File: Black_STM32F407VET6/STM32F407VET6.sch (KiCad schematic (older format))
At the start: 89 parts, among them J1 T0, J10 - HotBed +, J11 Heater0, J12 X-, J13 Y-, J14 Z-, J15 Z+, J16 USB_B, J17 LeftSpi, J18 EXTRAPINS, J19 12Vinput, J2 T1, J20 5VOut, J23 EXP2, J24 LCD2004, J25 Bottom, J26 Right, J28 LIGHTS, J29 Z, J3 TB, J30 Z, J38 X, J39 Y, J4 TC, J41 E0, J43 Heater1, J44 COM, J47 I2C, J48 SPI, J49 SPI, J5 + VIN -, J50 SDIO, J51 Servo, J52 Servo, J53 PowerSelect, J54 Power, J55 PD11, J56 Power, J6 Fan3, J7 Fan2, J8 Fan1, J9 Fan0, Q12 IRLR8726PBF, Q13 IRLR8726PBF, Q14 IRLR8726PBF, Q4 IRLML0030TRPBF, Q6 IRLML0030TRPBF, Q7 IRLML0030TRPBF, Q8 IRLML0030TRPBF, SW1 Boot0, U1 LeftAnalog, U2 Left5V, U3 BuckConvertor, U4 LM2901, U5 AT24CS01-SSHM, U6 LM2901

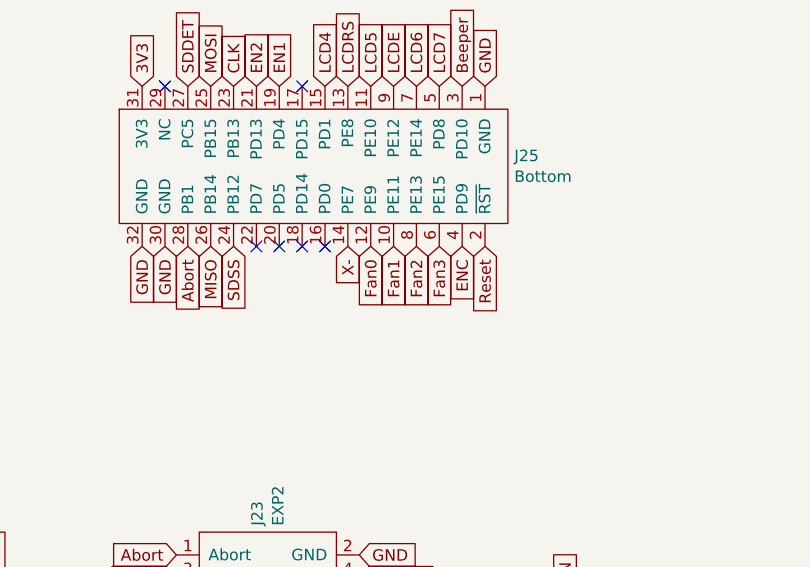
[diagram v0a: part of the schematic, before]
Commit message: Board layout with the opamps
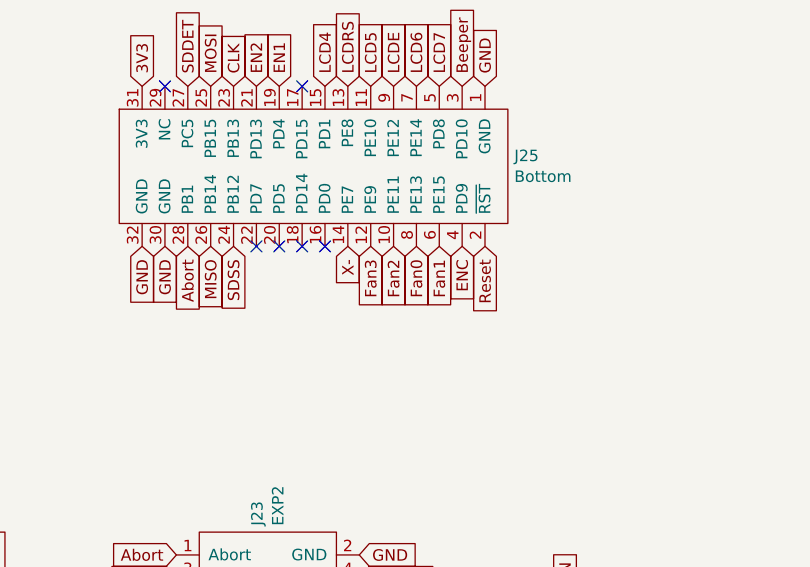
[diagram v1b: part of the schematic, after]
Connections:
- net Fan0: now also J25.8 (PE13); no longer J25.12 (PE9)
- net Fan1: now also J25.6 (PE15); no longer J25.10 (PE11)
- net Fan2: now also J25.10 (PE11); no longer J25.8 (PE13)
- net Fan3: now also J25.12 (PE9); no longer J25.6 (PE15)
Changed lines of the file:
@@
 EESchema Schematic File Version 4
 LIBS:STM32F407VET6-cache
-EELAYER 30 0
+EELAYER 29 0
 EELAYER END
 $Descr A3 16535 11693
@@
 Text GLabel 10700 4900 1    50   Input ~ 0
 3V3
+Text GLabel 11900 5600 3    50   Input ~ 0
+Fan0
+Text GLabel 12000 5600 3    50   Input ~ 0
+Fan1
+Text GLabel 11800 5600 3    50   Input ~ 0
+Fan2
 Text GLabel 11700 5600 3    50   Input ~ 0
-Fan0
-Text GLabel 11800 5600 3    50   Input ~ 0
-Fan1
-Text GLabel 11900 5600 3    50   Input ~ 0
-Fan2
-Text GLabel 12000 5600 3    50   Input ~ 0
 Fan3
 Text GLabel 11100 5600 3    50   Input ~ 0
